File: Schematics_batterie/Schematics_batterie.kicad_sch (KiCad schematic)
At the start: 6 parts, among them U2 MCP1802x-xx02xOT, U3 STM32G431KBTx

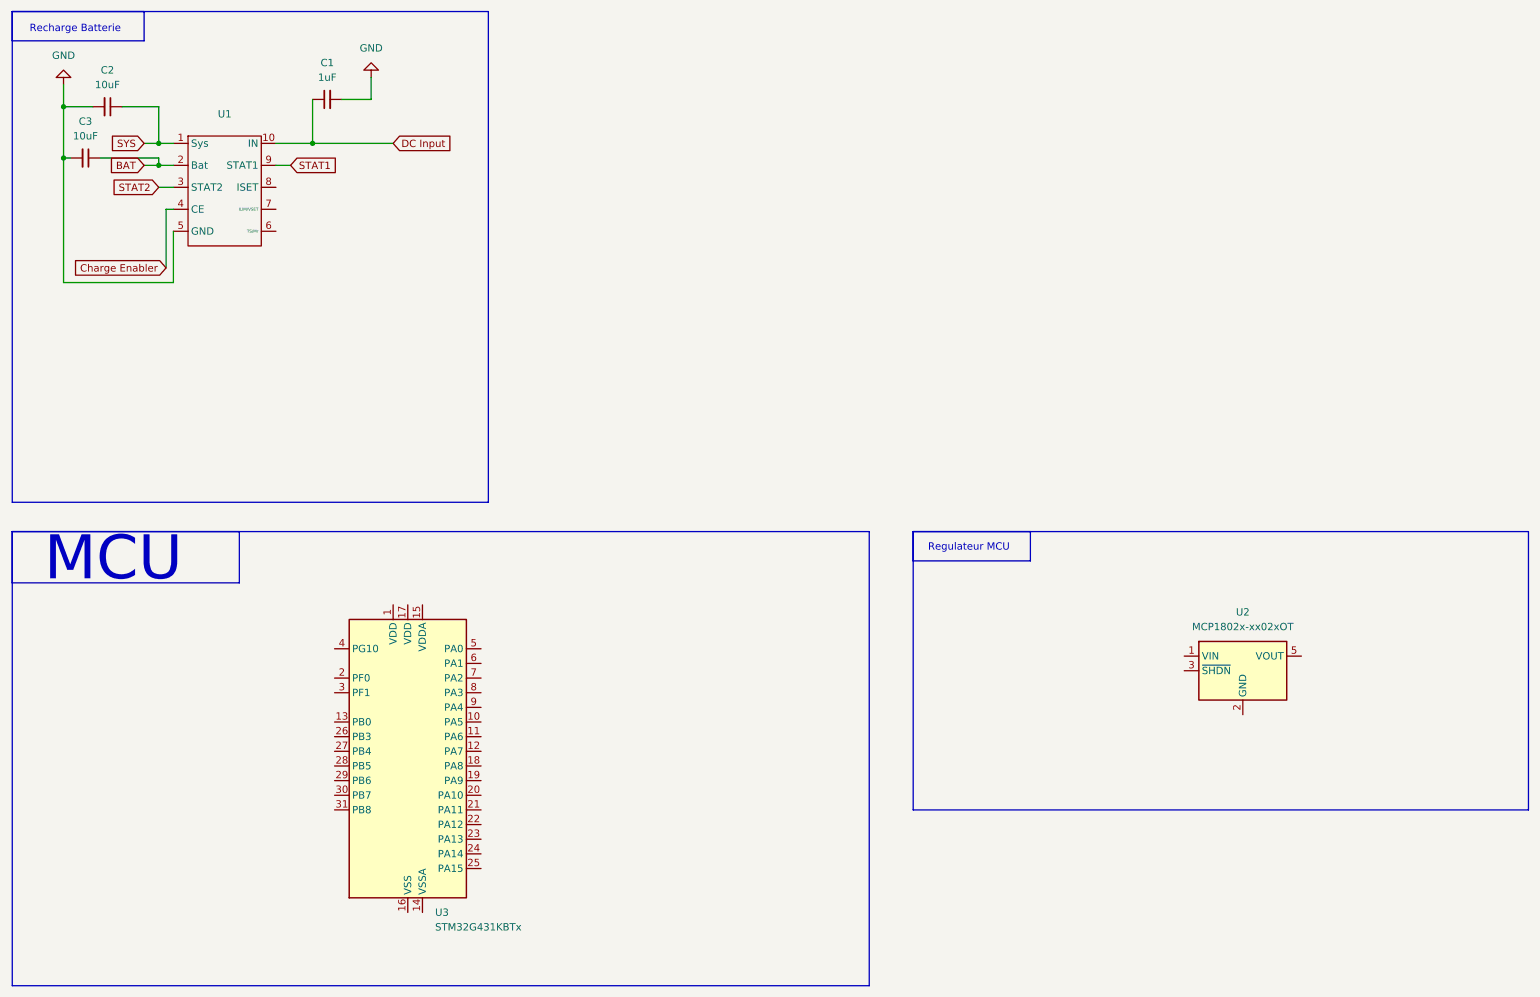
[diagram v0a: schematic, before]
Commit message: ok
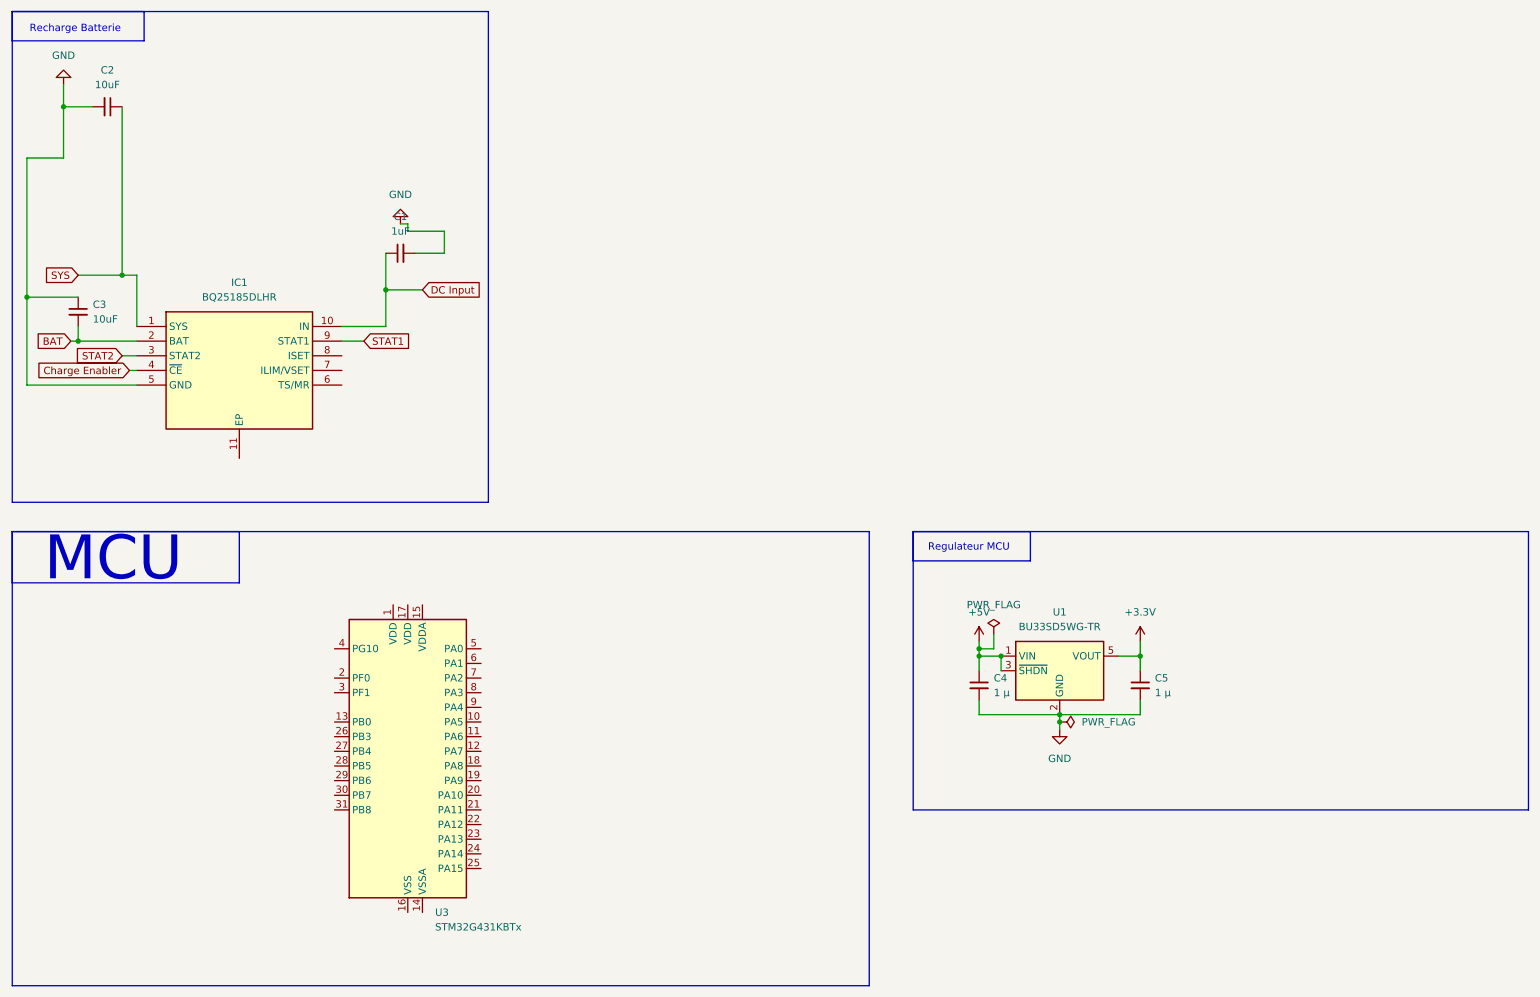
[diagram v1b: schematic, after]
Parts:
- removed U1: ~, symbol SamacSys_Parts:595-BQ25185DLHR
- removed U2: MCP1802x-xx02xOT, Package_TO_SOT_SMD:SOT-23-5, symbol Regulator_Linear:MCP1802x-xx02xOT
- added C4, C5: 1 µ, Capacitor_SMD:C_0603_1608Metric_Pad1.08x0.95mm_HandSolder, symbol Device:C_Small
- added IC1: BQ25185DLHR, SON40P220X200X80-11N, symbol BQ25185DLHR:BQ25185DLHR
- added U1: BU33SD5WG-TR, Package_TO_SOT_SMD:SOT-23-5, symbol Regulator_Linear:MCP1802x-xx02xOT
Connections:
- net BAT: now also C3.2, IC1.2 (BAT); no longer C3.1
- net Charge Enabler: now also IC1.4 (~{CE})
- net DC Input: now also IC1.10 (IN)
- net GND: now also C3.1, C4.2, C5.2, IC1.5 (GND), U1.2 (GND); no longer C3.2
- net STAT1: now also IC1.9 (STAT1)
- net STAT2: now also IC1.3 (STAT2)
- net SYS: now also IC1.1 (SYS)
- new net +3.3V: C5.1, U1.5 (VOUT)
- new net +5V: C4.1, U1.1 (VIN), U1.3 (~{SHDN})
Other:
- moved on the sheet: C1, C3
